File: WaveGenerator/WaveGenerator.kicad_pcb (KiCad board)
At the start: 2 copper layers, 37 parts, among them J1 Conn_01x05, J10 Conn_01x02, J2 Conn_01x06, J3 Conn_01x04, J4 USB_OTG, J5 VDD, SW1 SW_Rotary12, SW2 Rotary_Encoder, SW3 Rotary_Encoder, SW4 SW_Push_Dual, U1 AD9833, U2 PIC16F1459-ISS, U3 6N137, U4 LM7805_TO220, Y1 4MHz

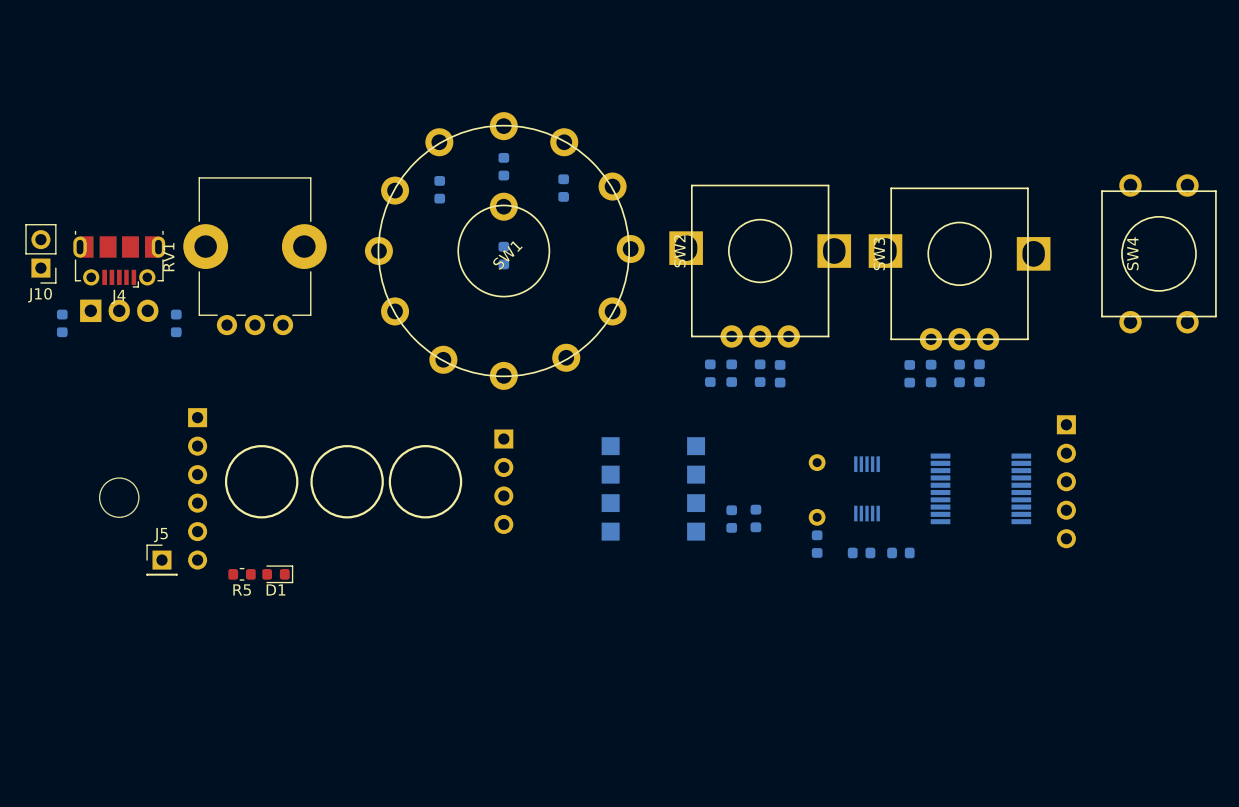
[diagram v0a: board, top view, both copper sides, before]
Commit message: Continued PCB wave
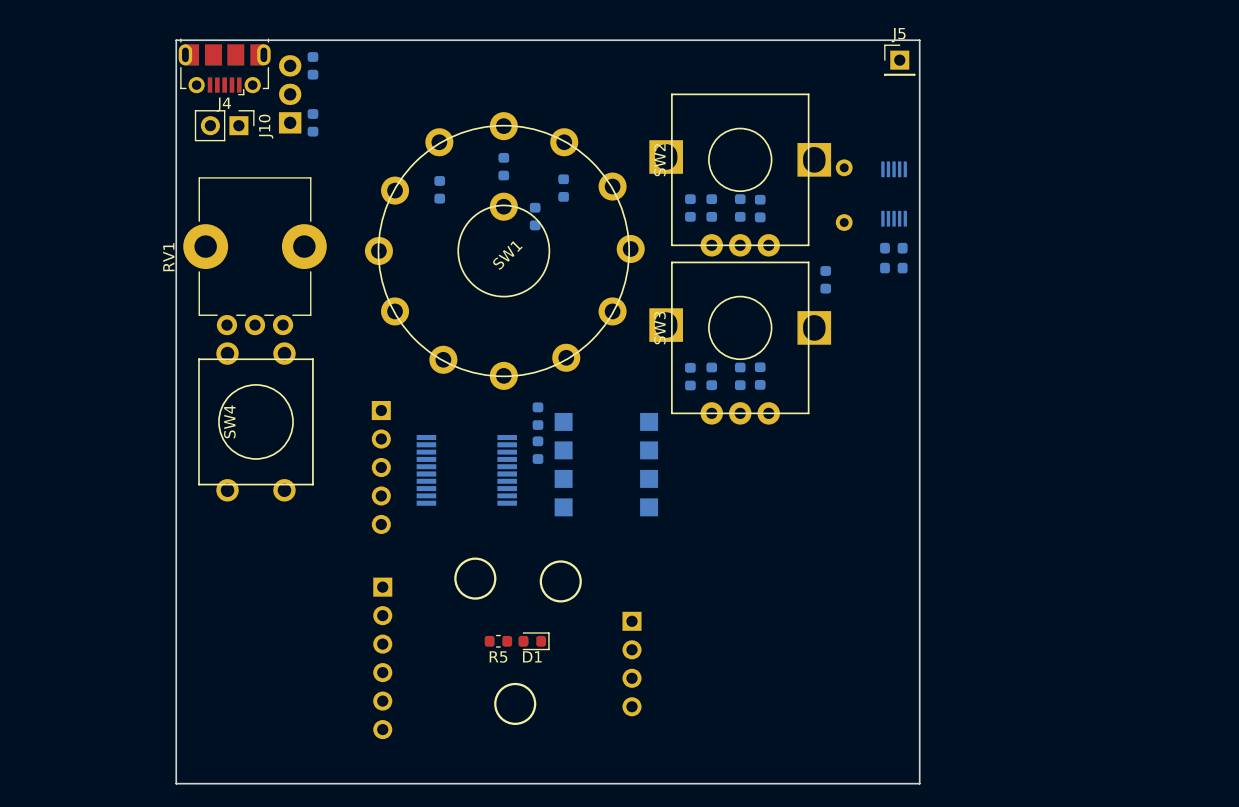
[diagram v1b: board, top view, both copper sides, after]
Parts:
- SW1: value SW_Rotary12 -> MODE
- SW2: value Rotary_Encoder -> D
- SW3: value Rotary_Encoder -> F
- SW4: value SW_Push_Dual -> TRIG
- U4: footprint Package_TO_SOT_THT:TO-220-3_Horizontal_TabDown -> Package_TO_SOT_THT:TO-220-3_Vertical
- moved SW4 81.9 mm to (135.4, 56.9)
- moved J5 79.5 mm to (192.8, 24.6)
- moved J1 61.1 mm to (146.6, 55.9)
- moved U2 45.9 mm to (154.2, 61.2)
- moved C10 28.6 mm to (140.5, 30.2), turned to 90 degrees
- moved C2 27.3 mm to (192.3, 41.4)
- moved U1 26.4 mm to (192.3, 36.6)
- moved Y1 26.4 mm to (187.8, 39.1)
- moved C11 26.0 mm to (140.5, 25.1)
- moved C1 25.4 mm to (192.3, 43.2)
- moved U4 24.4 mm to (138.4, 30.2), turned to 90 degrees
- moved D1 23.6 mm to (160.0, 76.5)
- moved R5 23.6 mm to (157.0, 76.5)
- moved C3 23.6 mm to (186.2, 44.2)
- moved J2 22.4 mm to (146.7, 71.6)
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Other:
- board outline added: 66.3 x 66.3 mm

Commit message: Wave gerber panelized
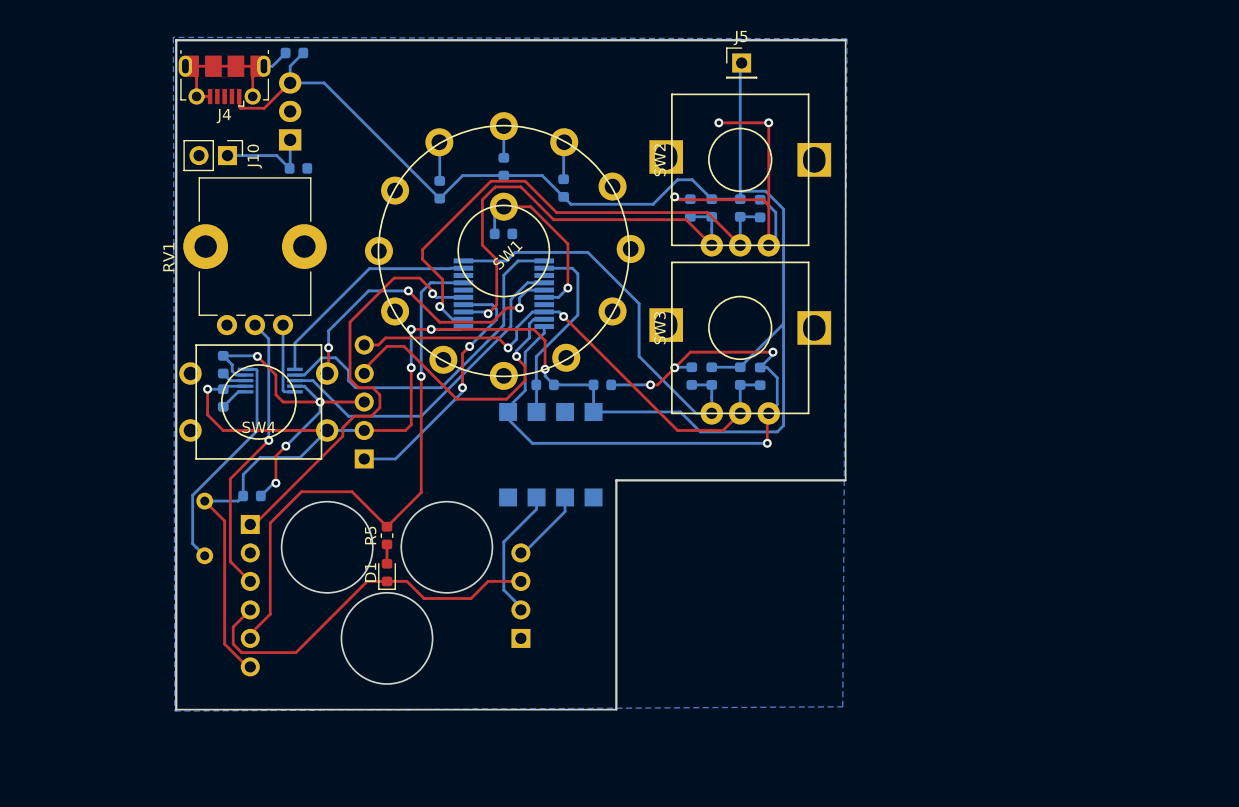
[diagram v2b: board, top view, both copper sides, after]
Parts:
- moved Y1 64.3 mm to (130.8, 68.8)
- moved C1 60.9 mm to (132.5, 54.8), turned to 90 degrees
- moved C2 60.7 mm to (132.5, 51.8), turned to 90 degrees
- moved U1 58.1 mm to (136.7, 53.2), turned to 0 degrees
- moved C3 54.7 mm to (135.0, 63.5), turned to 180 degrees
- moved U2 16.1 mm to (157.5, 45.5)
- moved D1 14.3 mm to (147.1, 70.3), turned to 90 degrees
- moved J5 14.1 mm to (178.7, 24.9)
- moved R5 13.7 mm to (147.1, 67.0), turned to 90 degrees
- moved J2 13.1 mm to (134.9, 66.0)
- moved J3 10.0 mm to (159.0, 76.2), turned to 0 degrees
- moved C4 6.38 mm to (166.3, 53.6), turned to 180 degrees
- moved R6 5.85 mm to (161.2, 53.6), turned to 0 degrees
- moved U3 5.03 mm to (161.7, 59.8), turned to 90 degrees
- moved J1 4.58 mm to (145.0, 60.2), turned to 0 degrees
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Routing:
- net VDD: track 0.00 -> 210.1 mm, vias 0 -> 5
- net BAT-: track 0.00 -> 172.6 mm, vias 0 -> 11
- net TRIGGER: track 0.00 -> 50.2 mm, vias 0 -> 1
- net B1: track 0.00 -> 46.1 mm, vias 0 -> 1
- net B2: track 0.00 -> 45.4 mm, vias 0 -> 2
- net A1: track 0.00 -> 40.8 mm, vias 0 -> 1
- net PWM: track 0.00 -> 38.6 mm, vias 0 -> 1
- net A2: track 0.00 -> 35.5 mm
- net SCK: track 0.00 -> 31.8 mm
- net FSYNC: track 0.00 -> 29.9 mm
- net Net-(SW4-Pad3): track 0.00 -> 27.4 mm, vias 0 -> 3
- net PGD: track 0.00 -> 25.5 mm, vias 0 -> 1
- net VOUT_: track 0.00 -> 25.5 mm, vias 0 -> 1
- net MCLR: track 0.00 -> 23.0 mm, vias 0 -> 2
- net Net-(U1-Pad5): track 0.00 -> 20.4 mm
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- added copper zone on B.Cu, net BAT-
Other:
- board size 66.3 x 66.3 mm -> 59.7 x 59.7 mm
